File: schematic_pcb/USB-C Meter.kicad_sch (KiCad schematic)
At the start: 11 parts, among them J1 USB_C_Receptacle_PowerOnly_6P, J2 USB_C_Receptacle_PowerOnly_6P, U1 WEMOS_D1_mini, U2 INA226, U3 Display I2C

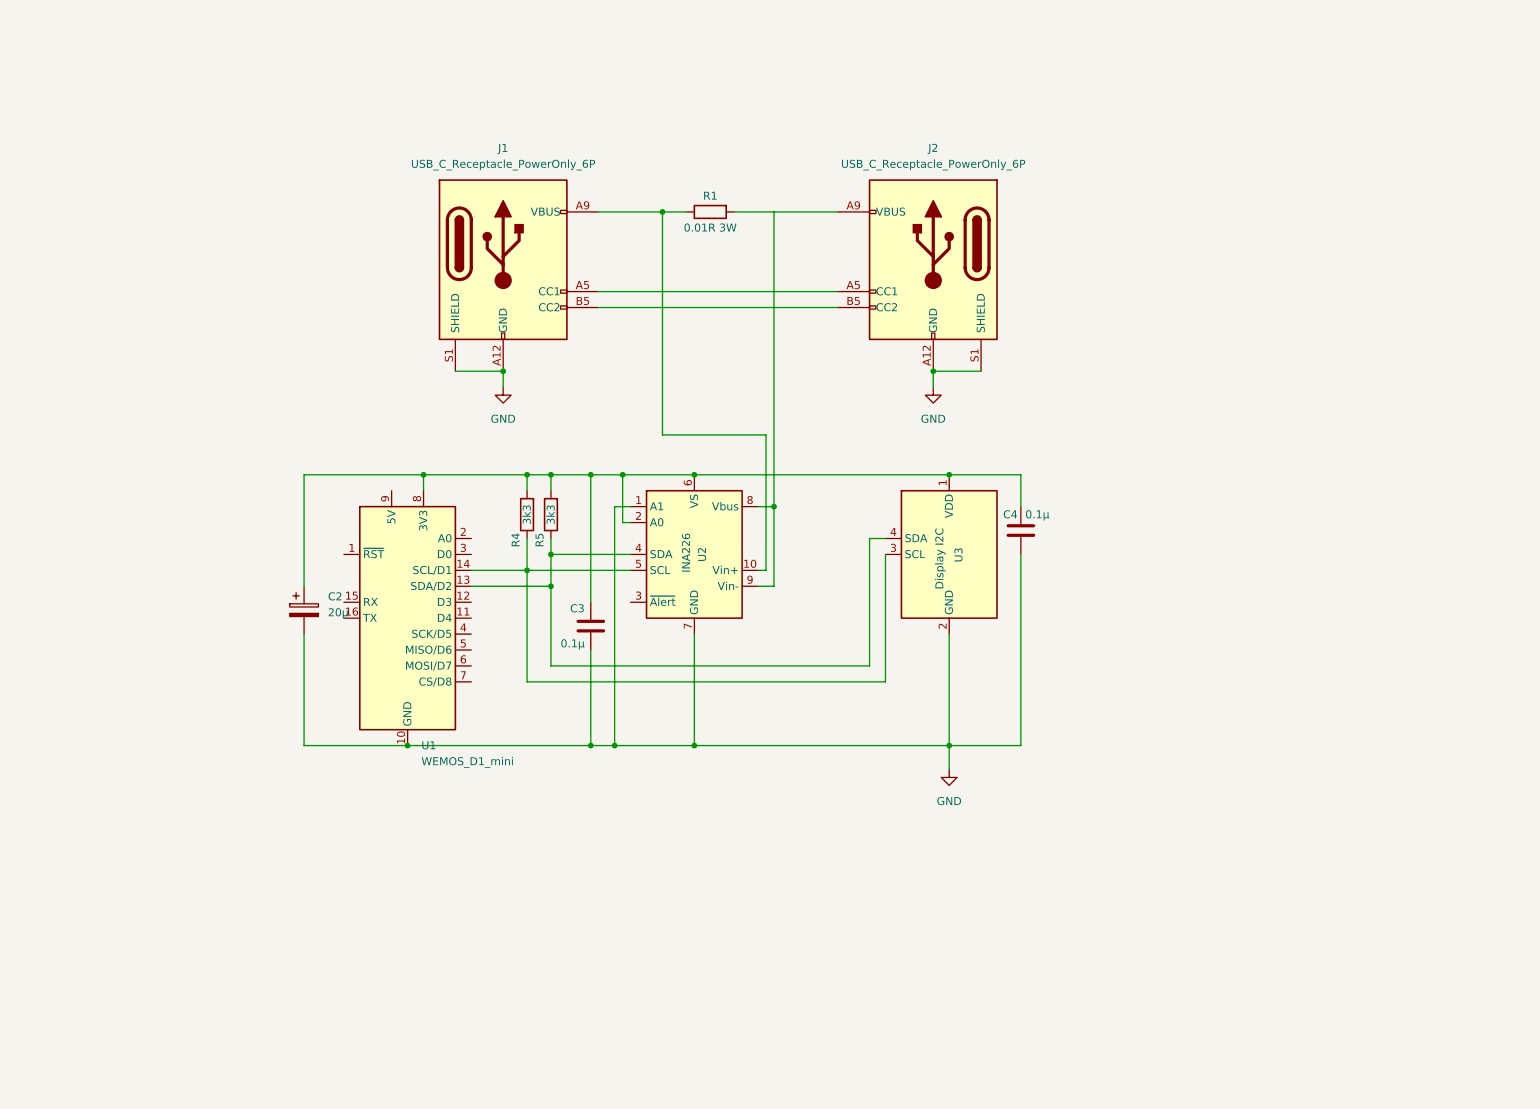
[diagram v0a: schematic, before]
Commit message: feat: pcb/schematic v2.1.0
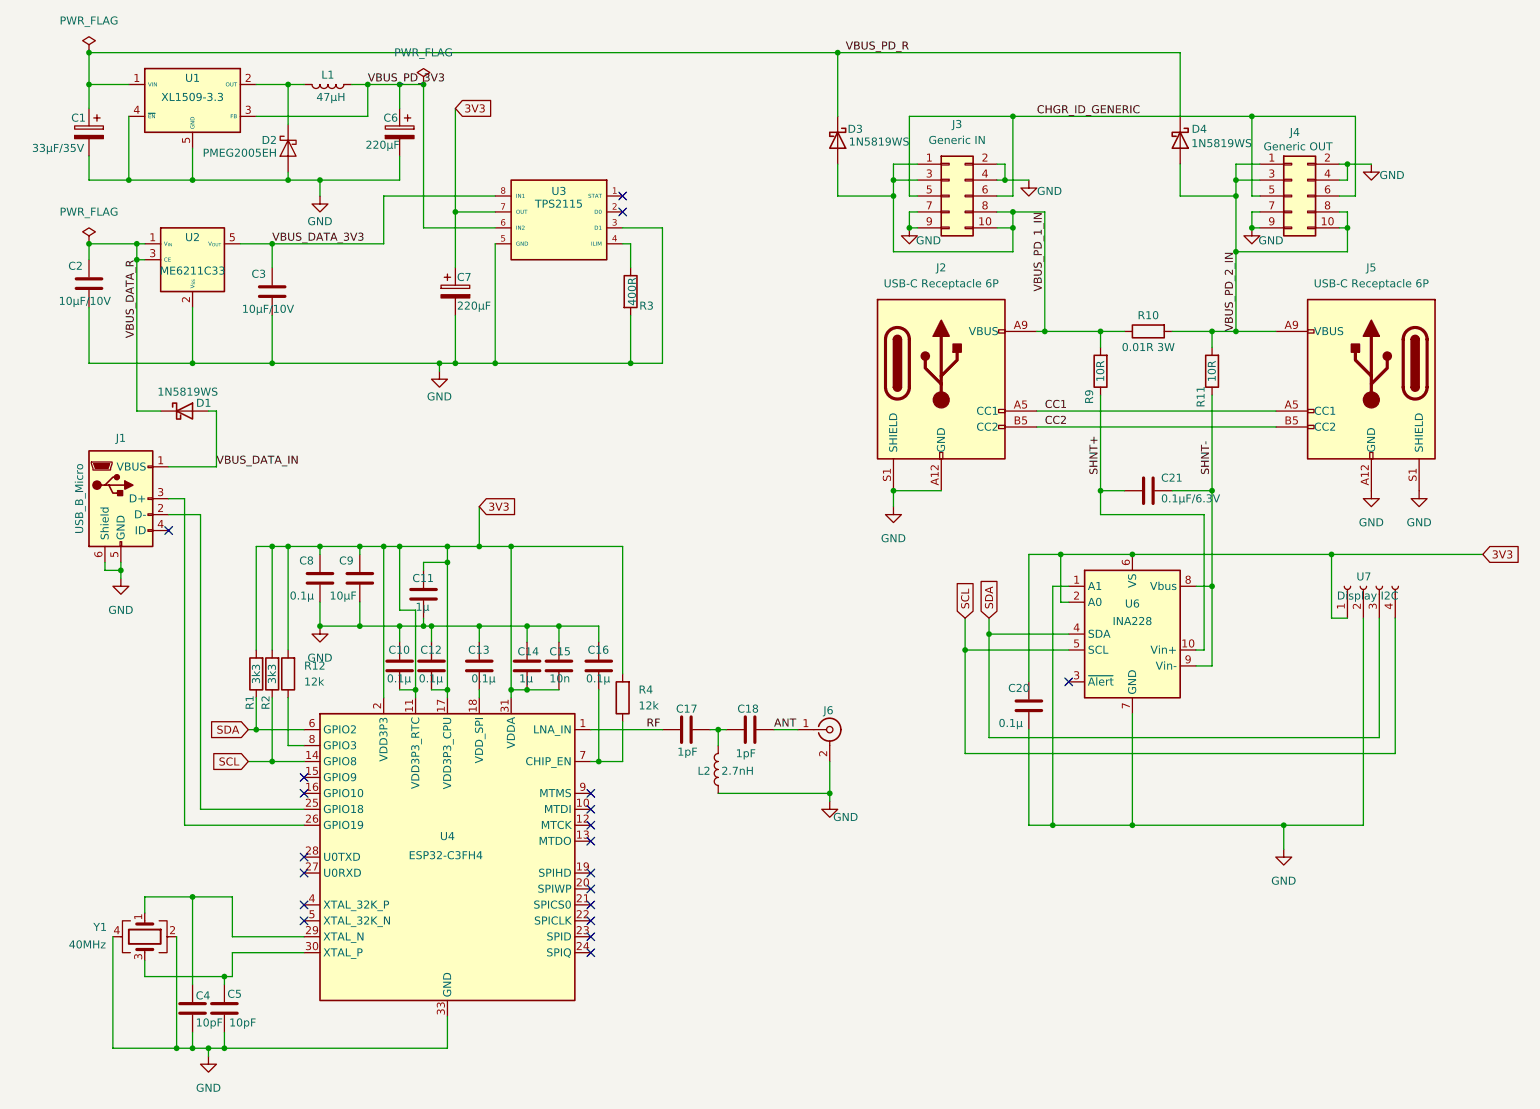
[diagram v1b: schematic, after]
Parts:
- removed C2: 20µ, Capacitor_Tantalum_SMD:CP_EIA-6032-20_AVX-F, symbol PCM_Capacitor_AKL:CP_SMD_Tantalum_AVX-F_6032
- removed U1: WEMOS_D1_mini, RF_Module:WEMOS_D1_mini_light, symbol RF_Module:WEMOS_D1_mini
- added C1: 33µF/35V, Capacitor_SMD:CP_Elec_5x5.8, symbol Device:C_Polarized
- added C10, C12, C13, C16, C8: 0.1µ, Capacitor_SMD:C_0603_1608Metric, symbol Device:C
- added C11, C14: 1µ, Capacitor_SMD:C_0603_1608Metric, symbol Device:C
- added C15: 10n, Capacitor_SMD:C_0603_1608Metric, symbol Device:C
- added C17, C18: 1pF, Capacitor_SMD:C_0402_1005Metric, symbol Device:C
- added C2, C3: 10µF/10V, Capacitor_SMD:C_0603_1608Metric, symbol Device:C
- added C21: 0.1µF/6.3V, Capacitor_SMD:C_0603_1608Metric, symbol Device:C
- added C5: 10pF, Capacitor_SMD:C_0402_1005Metric, symbol Device:C
- added C6, C7: 220µF, Capacitor_SMD:CP_Elec_6.3x5.9, symbol Device:C_Polarized
- added C9: 10µF, Capacitor_SMD:C_0603_1608Metric, symbol Device:C
- added D1, D3, D4: 1N5819WS, Diode_SMD:D_SOD-323, symbol Diode:1N5819WS
- added D2: PMEG2005EH, Diode_SMD:D_SOD-123F, symbol Diode:PMEG2005EH
- added J1: USB_B_Micro, Connector_USB:USB_Micro-B_Wuerth_629105150521, symbol Connector:USB_B_Micro
- added J3: Generic IN, Connector_PinHeader_2.54mm:PinHeader_2x05_P2.54mm_Horizontal, symbol Connector_Generic:Conn_02x05_Odd_Even
- added J4: Generic OUT, Connector_PinSocket_2.54mm:PinSocket_2x05_P2.54mm_Horizontal, symbol Connector_Generic:Conn_02x05_Odd_Even
- added J6: Conn_Coaxial, Connector_Coaxial:U.FL_Hirose_U.FL-R-SMT-1_Vertical, symbol Connector:Conn_Coaxial
- added L1: 47µH, Inductor_SMD:L_Changjiang_FXL0630, symbol Device:L
- added L2: 2.7nH, Inductor_SMD:L_0603_1608Metric_Pad1.05x0.95mm_HandSolder, symbol Device:L
- added R11, R9: 10R, Resistor_SMD:R_0402_1005Metric, symbol Device:R
- added R12, R4: 12k, Resistor_SMD:R_0603_1608Metric_Pad0.98x0.95mm_HandSolder, symbol Device:R
- added R3: 400R, Resistor_SMD:R_0402_1005Metric, symbol Device:R
- added U1: XL1509-3.3, Package_SO:SOIC-8_3.9x4.9mm_P1.27mm, symbol Regulator_Switching:XL1509-3.3
- added U2: ME6211C33, Package_TO_SOT_SMD:SOT-23-5, symbol Regulator_Linear:ME6211C33M5
- added U3: TPS2115, Package_SO:TSSOP-8_4.4x3mm_P0.65mm, symbol TPS2115:TPS2115
- added U4: ESP32-C3FH4, Package_DFN_QFN:QFN-32-1EP_5x5mm_P0.5mm_EP3.7x3.7mm, symbol MCU_Espressif:ESP32-C3
- added Y1: 40MHz, Crystal:Crystal_SMD_3225-4Pin_3.2x2.5mm, symbol Device:Crystal_GND24
- C4: value 0.1µ -> 10pF; footprint Capacitor_SMD:C_0603_1608Metric -> Capacitor_SMD:C_0402_1005Metric
- J2: renamed from J1; value USB_C_Receptacle_PowerOnly_6P -> USB-C Receptacle 6P; footprint Connector_USB:USB_C_Receptacle_HRO_TYPE-C-31-M-17 -> Connector_USB:USB_C_Receptacle_GCT_USB4125-xx-x_6P_TopMnt_Horizontal
- J5: renamed from J2; value USB_C_Receptacle_PowerOnly_6P -> USB-C Receptacle 6P
- R10: renamed from R1; footprint Resistor_SMD:R_1206_3216Metric -> Resistor_SMD:R_2512_6332Metric
- U6: renamed from U2; value INA226 -> INA228
- U7: renamed from U3; footprint Connector_PinHeader_2.54mm:PinHeader_1x04_P2.54mm_Vertical -> Connector_PinSocket_2.54mm:PinSocket_1x04_P2.54mm_Vertical; symbol Display_Character:NHD-C0220BIZ -> Connector:Conn_01x04_Socket
- renumbered C3 to C20, R5 to R1, R4 to R2
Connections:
- net GND: now also C4.2, C1.2, C10.1, C11.2, C12.1, C13.1, C14.1, C15.1, C16.1, C2.2, C3.2, C5.1, C6.2, C7.2, C8.2, C9.2, D2.2 (A), J1.5 (GND), J1.6 (Shield), J3.2 (Pin_2), J3.4 (Pin_4), J3.7 (Pin_7), J3.9 (Pin_9), J4.2 (Pin_2), J4.4 (Pin_4), J4.7 (Pin_7), J4.9 (Pin_9), J6.2 (Ext), L2.1, R3.2, U1.4 (~{EN}), U1.5 (GND), U1.6 (GND), U1.7 (GND), U1.8 (GND), U2.2 (V_{SS}), U3.3 (D1), U3.5 (GND), U4.33 (GND), Y1.2, Y1.4; no longer C4.1
- net VBUS_PD_1_IN: now reaches J2.A9 (VBUS), J2.B9 (VBUS), R10.1
- net VBUS_PD_1_IN: now also D3.2 (A), J3.1 (Pin_1), J3.10 (Pin_10), J3.3 (Pin_3), J3.8 (Pin_8), R9.2; no longer U6.10 (Vin+)
- net 3V3: now reaches C20.1, R1.2, R2.2, U6.2 (A0), U6.6 (VS), U7.1 (Pin_1)
- net 3V3: now also C10.2, C11.1, C12.2, C14.2, C15.2, C7.1, C8.1, C9.1, R12.2, R4.2, U3.7 (OUT), U4.11 (VDD3P3_RTC), U4.17 (VDD3P3_CPU), U4.2 (VDD3P3), U4.3 (VDD3P3), U4.31 (VDDA), U4.32 (VDDA); no longer C4.2
- net SDA: now reaches R1.1, U6.4 (SDA)
- net SDA: now also U7.3 (Pin_3), U4.6 (GPIO2); no longer U7.4 (SDA)
- net SCL: now reaches R2.1, U6.5 (SCL)
- net SCL: now also U7.4 (Pin_4), U4.14 (GPIO8); no longer U7.3 (SCL)
- net SHNT-: now reaches U6.8 (Vbus), U6.9 (Vin-)
- net SHNT-: now also C21.2, R11.1
- net CC1: now reaches J2.A5 (CC1), J5.A5 (CC1)
- net VBUS_PD_2_IN: now reaches J5.A9 (VBUS), J5.B9 (VBUS), R10.2
- net VBUS_PD_2_IN: now also D4.2 (A), J4.1 (Pin_1), J4.10 (Pin_10), J4.3 (Pin_3), J4.8 (Pin_8), R11.2
- net CC2: now reaches J2.B5 (CC2), J5.B5 (CC2)
- new net: C16.2, R4.1, U4.7 (CHIP_EN)
- new net: J1.2 (D-), U4.25 (GPIO18)
- new net: J1.3 (D+), U4.26 (GPIO19)
- new net: C4.1, U4.29 (XTAL_N), Y1.1
- new net: C17.2, C18.2, L2.2
- new net: D2.1 (K), L1.1, U1.2 (OUT)
- new net: C13.2, U4.18 (VDD_SPI)
- new net: C5.2, U4.30 (XTAL_P), Y1.3
- new net: R12.1, U4.8 (GPIO3)
- new net: R3.1, U3.4 (ILIM)
- new net ANT: C18.1, J6.1 (In)
- new net CHGR_ID_GENERIC: J3.5 (Pin_5), J3.6 (Pin_6), J4.5 (Pin_5), J4.6 (Pin_6)
- new net RF: C17.1, U4.1 (LNA_IN)
- new net SHNT+: C21.1, R9.1, U6.10 (Vin+)
- new net VBUS_DATA_3V3: C3.1, U2.5 (V_{OUT}), U3.8 (IN1)
- new net VBUS_DATA_IN: D1.2 (A), J1.1 (VBUS)
- new net VBUS_DATA_R: C2.1, D1.1 (K), U2.1 (V_{IN}), U2.3 (CE)
- new net VBUS_PD_3V3: C6.1, L1.2, U1.3 (FB), U3.6 (IN2)
- new net VBUS_PD_R: C1.1, D3.1 (K), D4.1 (K), U1.1 (VIN)
- no-connect marks 0 -> 20
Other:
- company: Netwake -> Macwake.de
- moved on the sheet: C20, J2, J5, R1, R10, R2, U6

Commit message: feat: pcb/schematic v2.1.1
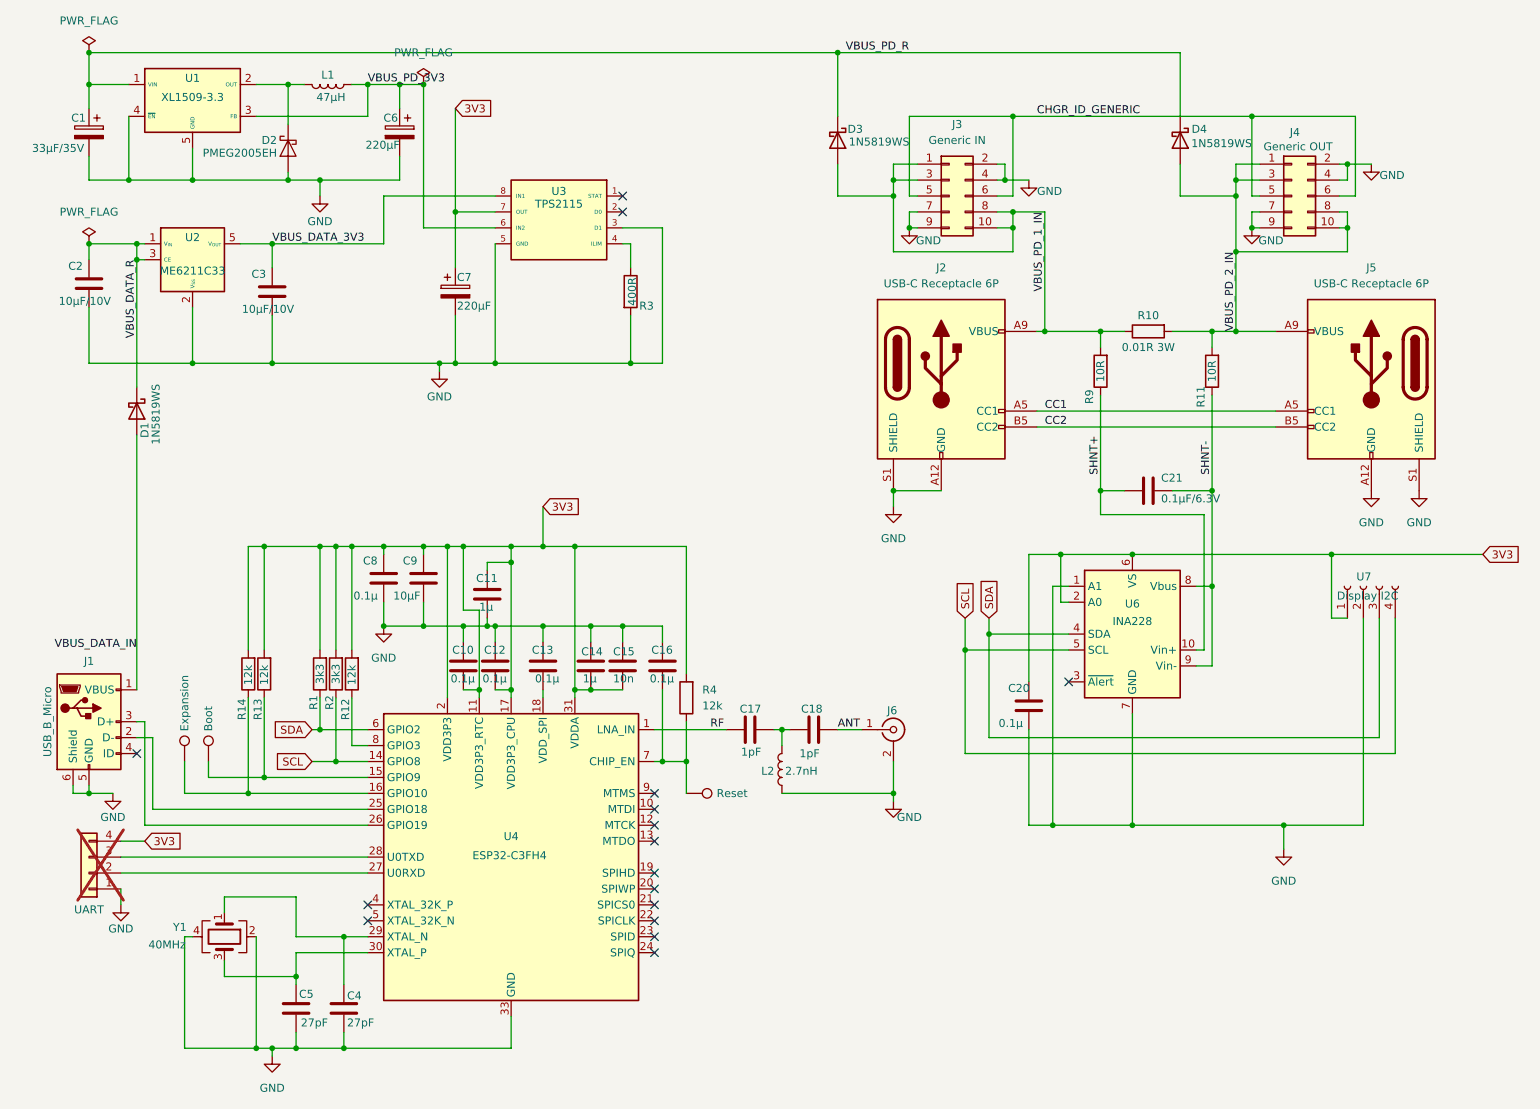
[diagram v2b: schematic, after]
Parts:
- added J7: UART, Connector_PinHeader_1.00mm:PinHeader_1x04_P1.00mm_Vertical_SMD_Pin1Left, symbol Connector_Generic:Conn_01x04
- added R13, R14: 12k, Resistor_SMD:R_0603_1608Metric_Pad0.98x0.95mm_HandSolder, symbol Device:R
- added TP1: Boot, TestPoint:TestPoint_Pad_D1.5mm, symbol Connector:TestPoint
- added TP2: Expansion, TestPoint:TestPoint_Pad_D1.5mm, symbol Connector:TestPoint
- added TP3: Reset, TestPoint:TestPoint_Pad_D1.5mm, symbol Connector:TestPoint
- C4, C5: value 10pF -> 27pF
- D1, D3, D4: footprint Diode_SMD:D_SOD-323 -> Diode_SMD:D_SOD-123F
- R1, R2: footprint Resistor_SMD:R_0402_1005Metric -> Resistor_SMD:R_0603_1608Metric_Pad0.98x0.95mm_HandSolder
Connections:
- net 3V3: now also J7.4 (Pin_4), R13.2, R14.2
- net GND: now also J7.1 (Pin_1)
- net at C16.2, R4.1, U4.7 (CHIP_EN): now also TP3.1
- net at U4.15 (GPIO9): now also R13.1, TP1.1
- net at U4.16 (GPIO10): now also R14.1, TP2.1
- net at U4.27 (U0RXD): now also J7.2 (Pin_2)
- net at U4.28 (U0TXD): now also J7.3 (Pin_3)
- no-connect marks 20 -> 16
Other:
- moved on the sheet: C10, C11, C12, C13, C14, C15, C16, C17, C18, C4, C5, C8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
